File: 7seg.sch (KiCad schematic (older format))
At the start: 12 parts, among them J1 Conn_01x05, J2 Conn_01x05, U1 74HC595, U2 HDSP-7401

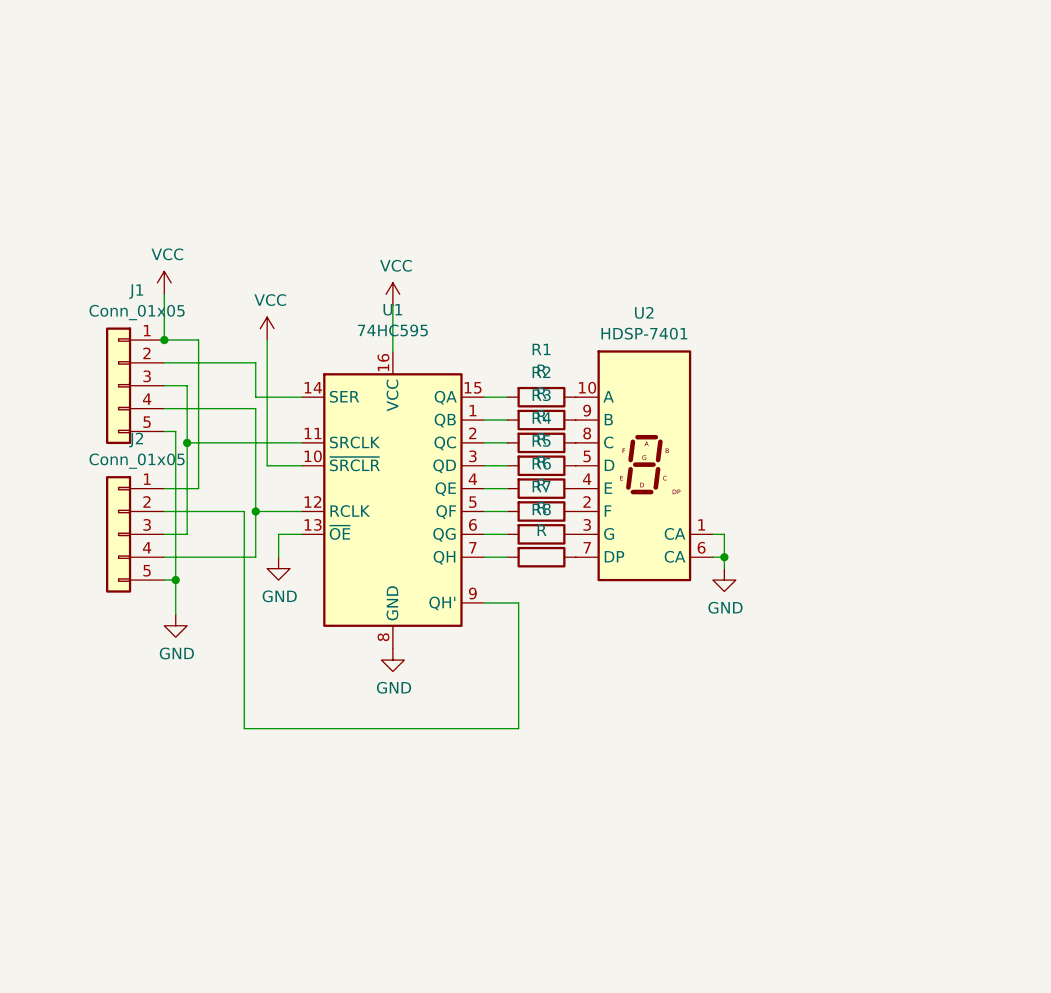
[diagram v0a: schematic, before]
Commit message: Add files via upload
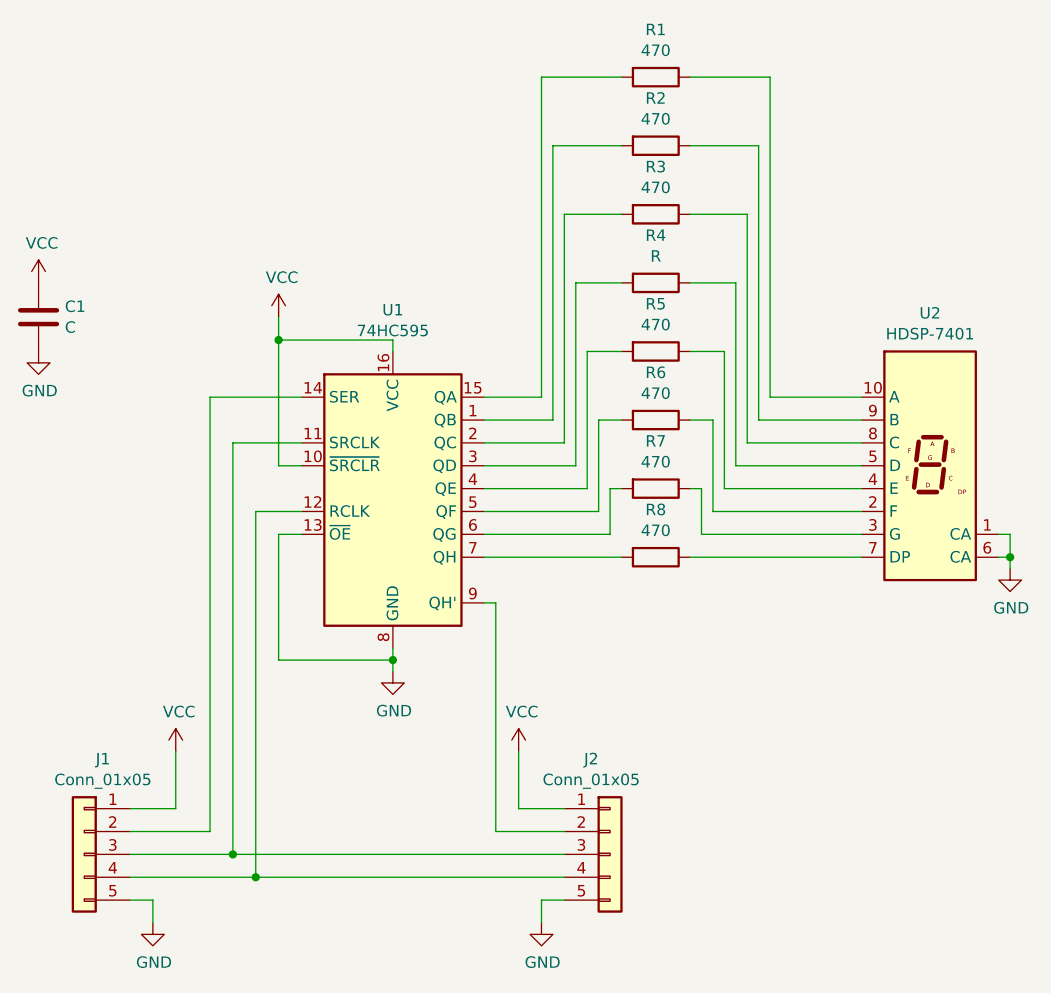
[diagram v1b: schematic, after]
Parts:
- added C1: C, Capacitors_SMD:C_0402, symbol Device:C
- R1, R2, R3, R5, R6, R7, R8: value R -> 470
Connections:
- net GND: now also C1.2
- net VCC: now also C1.1
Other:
- moved on the sheet: J1, J2, R1, R2, R3, R4, R5, R6, R7, R8, U2
